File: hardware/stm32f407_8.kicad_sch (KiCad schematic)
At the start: 28 parts, among them J10 Conn_01x04, J8 USB_B_Mini, J9 Conn_01x04, SW3 SW TACT-SPST, U7 STM32F407VGT6, Y3 ABM8G-8.000MHZ-18-D2Y-T

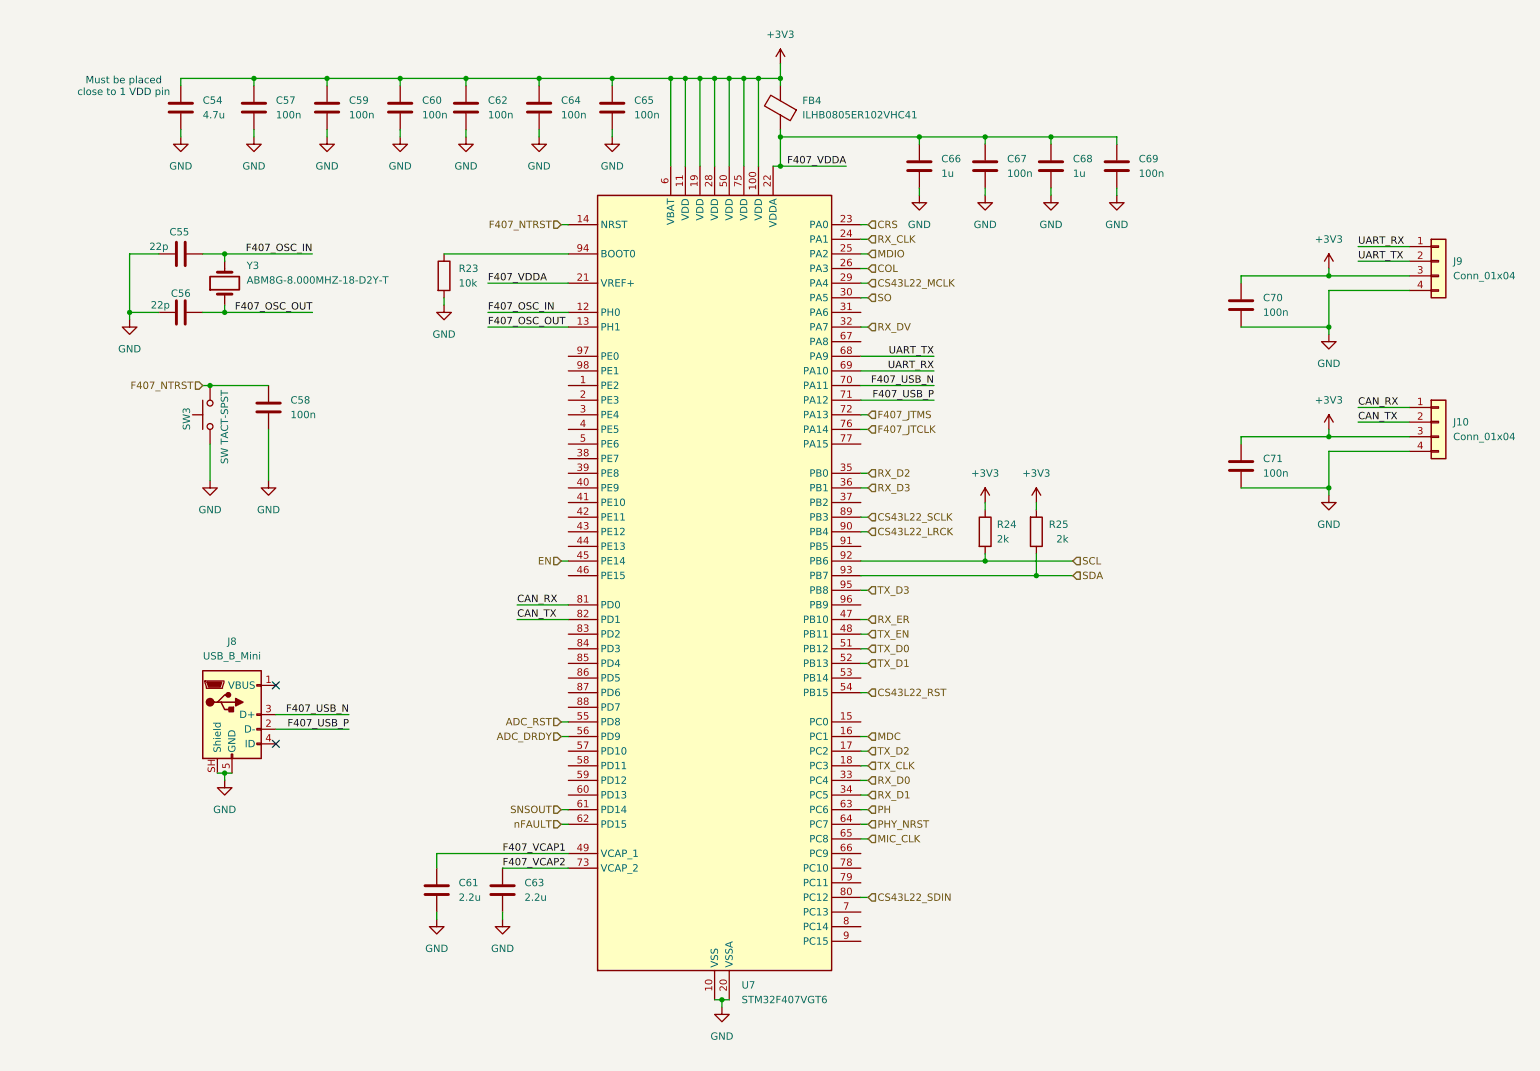
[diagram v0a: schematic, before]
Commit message: Organize schematic
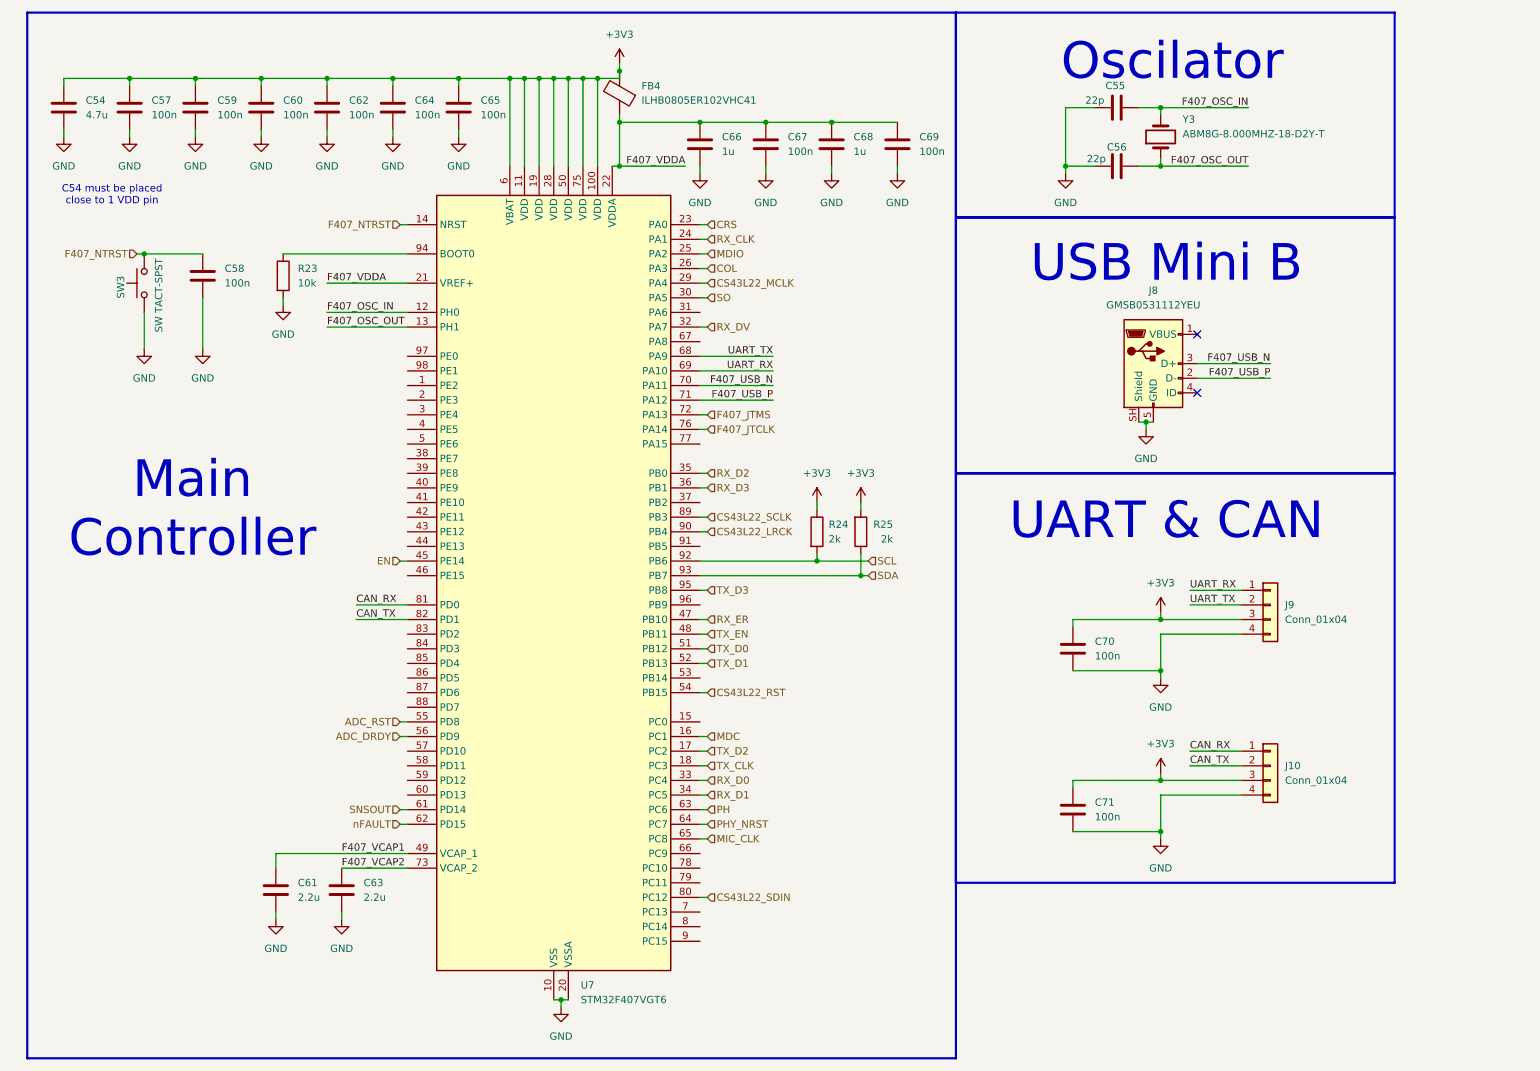
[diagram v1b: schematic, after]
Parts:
- J8: value USB_B_Mini -> GMSB0531112YEU
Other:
- note added: "C54 must be placed close to 1 VDD pin"
- note added: "Main Controller"
- note added: "Oscilator"
- note added: "UART & CAN"
- note added: "USB Mini B"
- note removed: "Must be placed close to 1 VDD pin"
- moved on the sheet: C54, C55, C56, C57, C58, C59, C60, C61, C62, C63, C64, C65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
